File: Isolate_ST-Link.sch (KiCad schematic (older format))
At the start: 55 parts, among them J2 Conn_02x05_Odd_Even, J3 CONN_01X04, J4 CONN_01X02, J5 CONN_01X02, J7 USB_C_Receptacle_USB2.0, Q1 BSS138, U1 RFM-0505S, U2 ADuM4160, U3 APE8865NR-33-HF-3

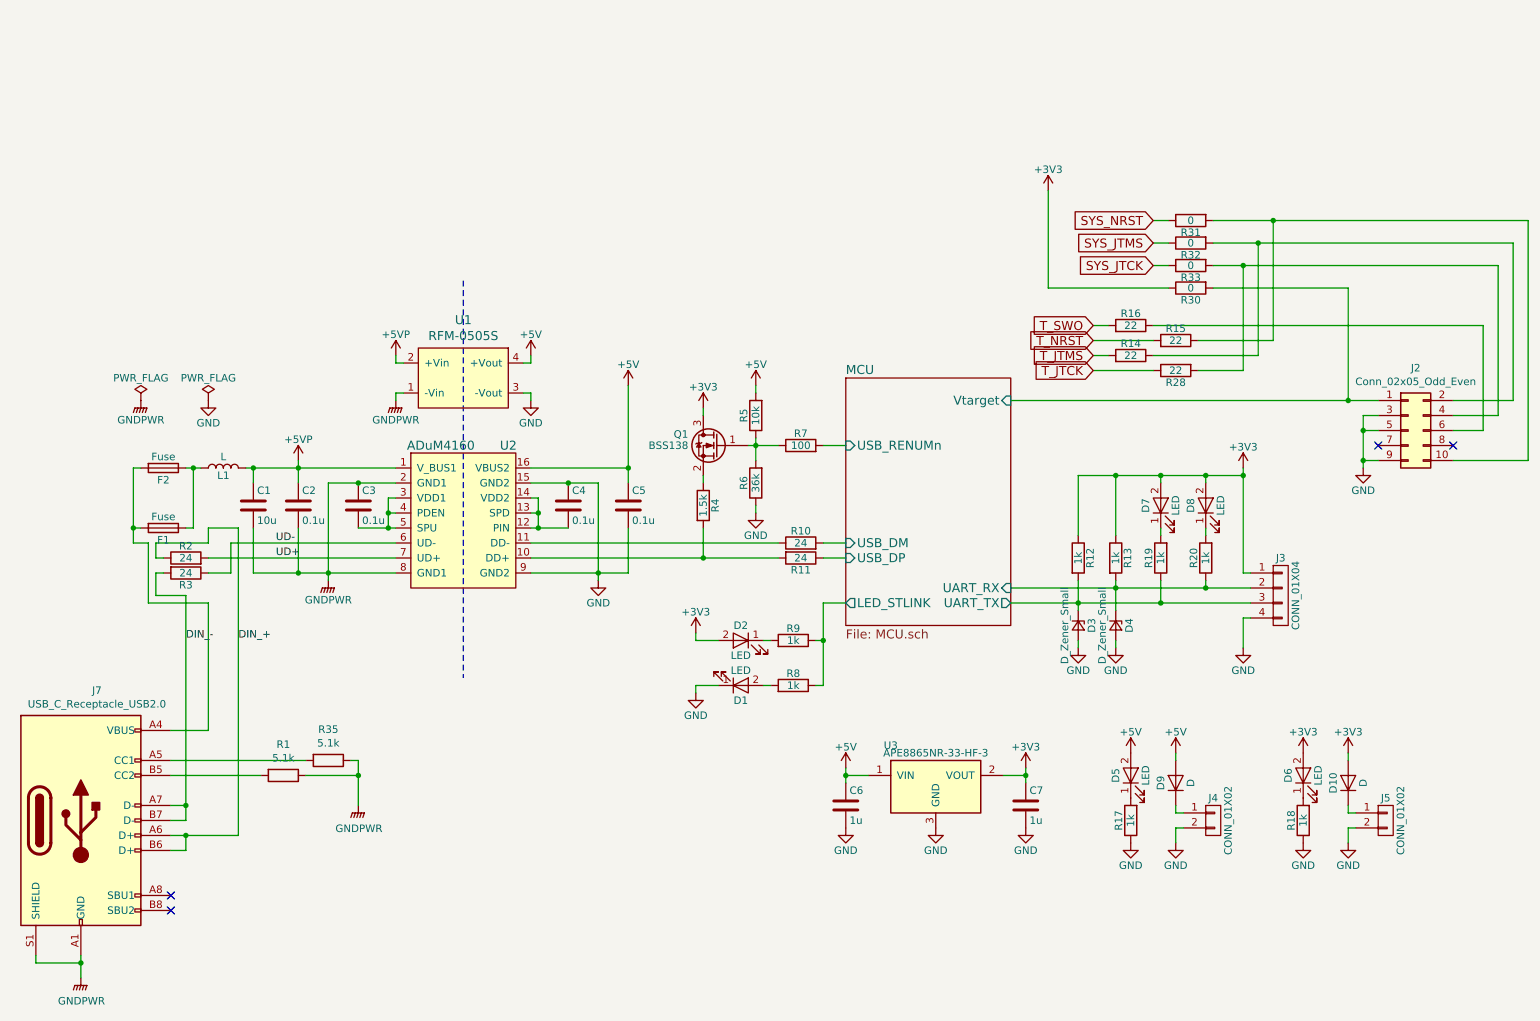
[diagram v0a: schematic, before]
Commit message: 整理
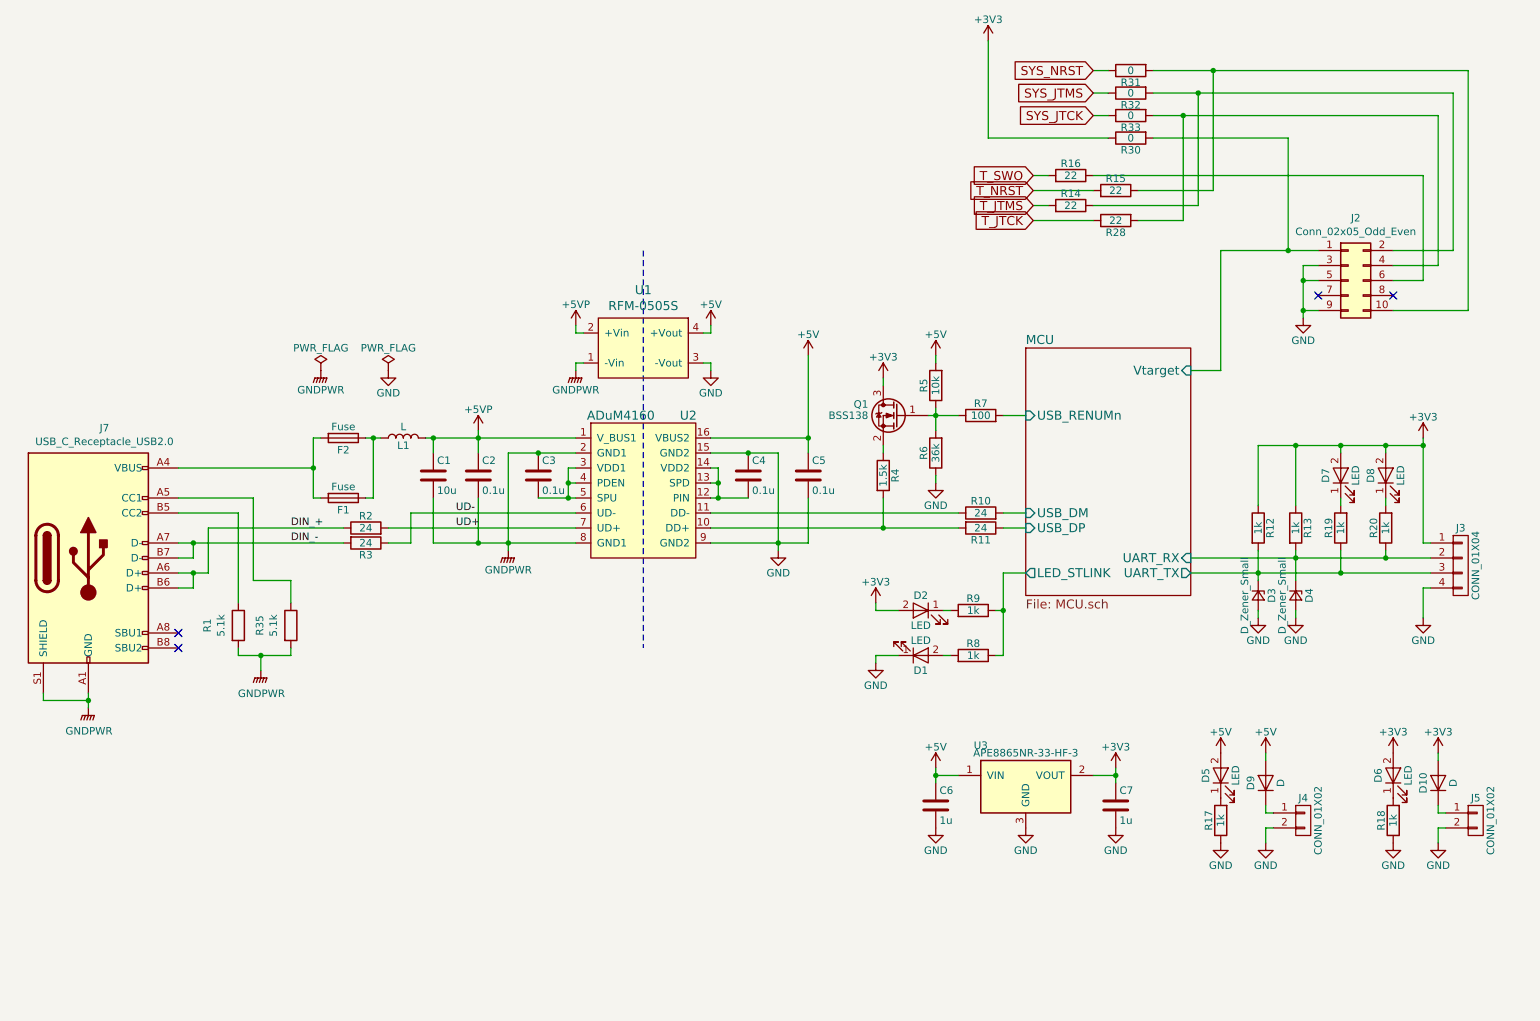
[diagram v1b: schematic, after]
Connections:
- net GNDPWR: now also R1.2, R35.2; no longer R1.1, R35.1
- net at J7.A5 (CC1): now also R35.1; no longer R35.2
- net at J7.B5 (CC2): now also R1.1; no longer R1.2
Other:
- moved on the sheet: C1, C2, C3, C4, C5, C6, C7, D1, D10, D2, D3, D4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
